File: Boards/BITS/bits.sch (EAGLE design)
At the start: 39 parts, among them T1 Si1013, U1 LMR16020, X1 22-23-2021, X2 53398-10, X3 22-23-2031, X4 22-23-2041

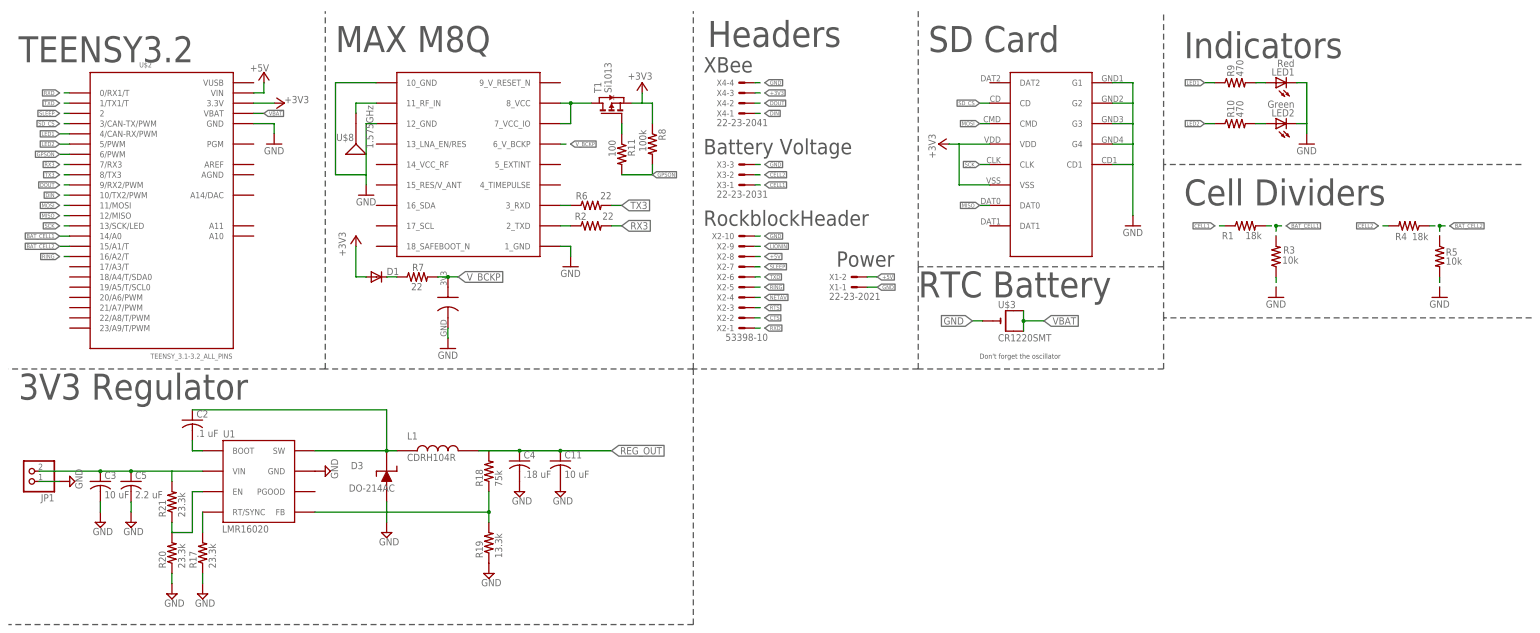
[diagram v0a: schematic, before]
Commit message: Revert "reverted bits schematic back to my last commit""
This reverts commit d8380e26c9c134d67ee78542be9b2ca2b8e420f0.
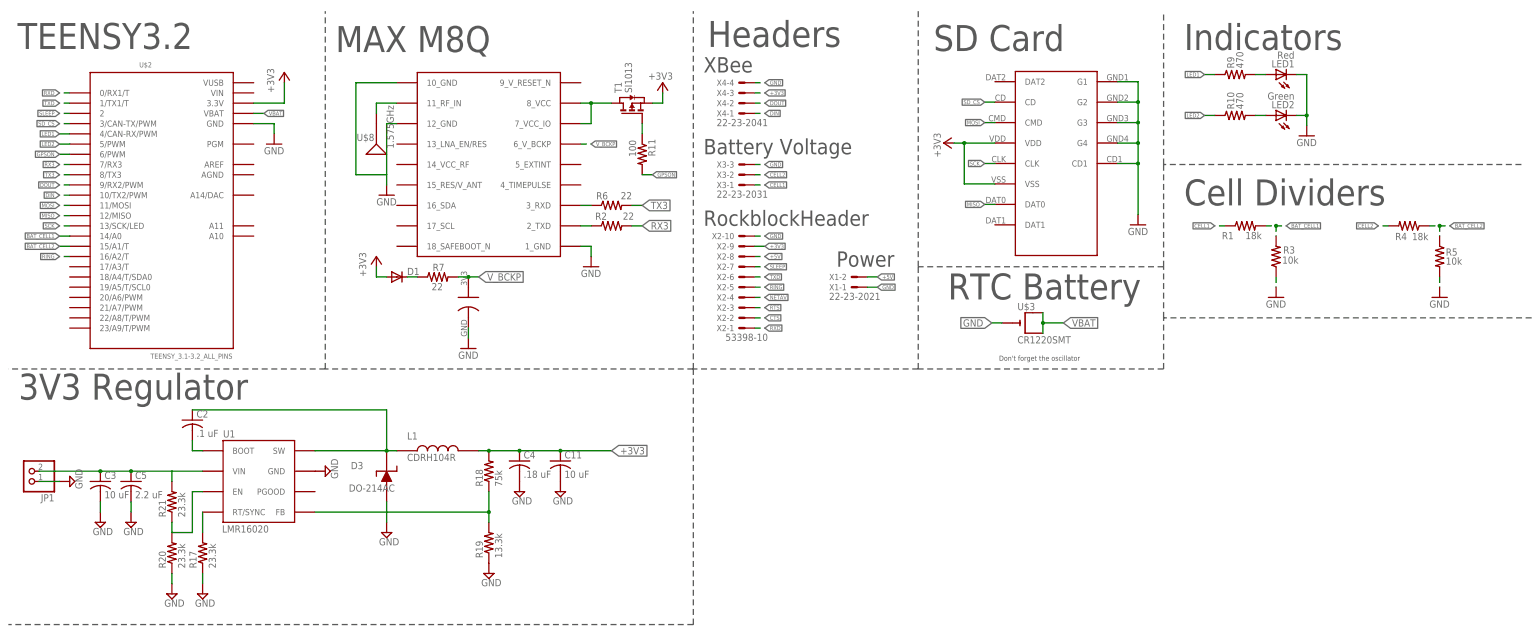
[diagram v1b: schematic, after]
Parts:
- removed R8: 100k, rcl:R-US_R0603
- T1: value Si1013 -> SI1013; device zetex:PMOSSOT23 -> cmdLibs:SI1013; SPICEPREFIX J -> (none)
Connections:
- removed net LIONIN: X2-9.S
- removed net REG_OUT: C11.1, C4.1, L1.P$2, R18.2
- net +3V3: now also C11.1, C4.1, L1.P$2, R18.2, X2-9.S; no longer R8.1
- net +5V: no longer U$2.VIN
- net GPSON: no longer R8.2
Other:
- moved on the sheet: D1, LED1, LED2, R10, R11, R2, R6, R7, R9, U$3, U$8
